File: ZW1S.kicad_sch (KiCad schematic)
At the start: 0 parts

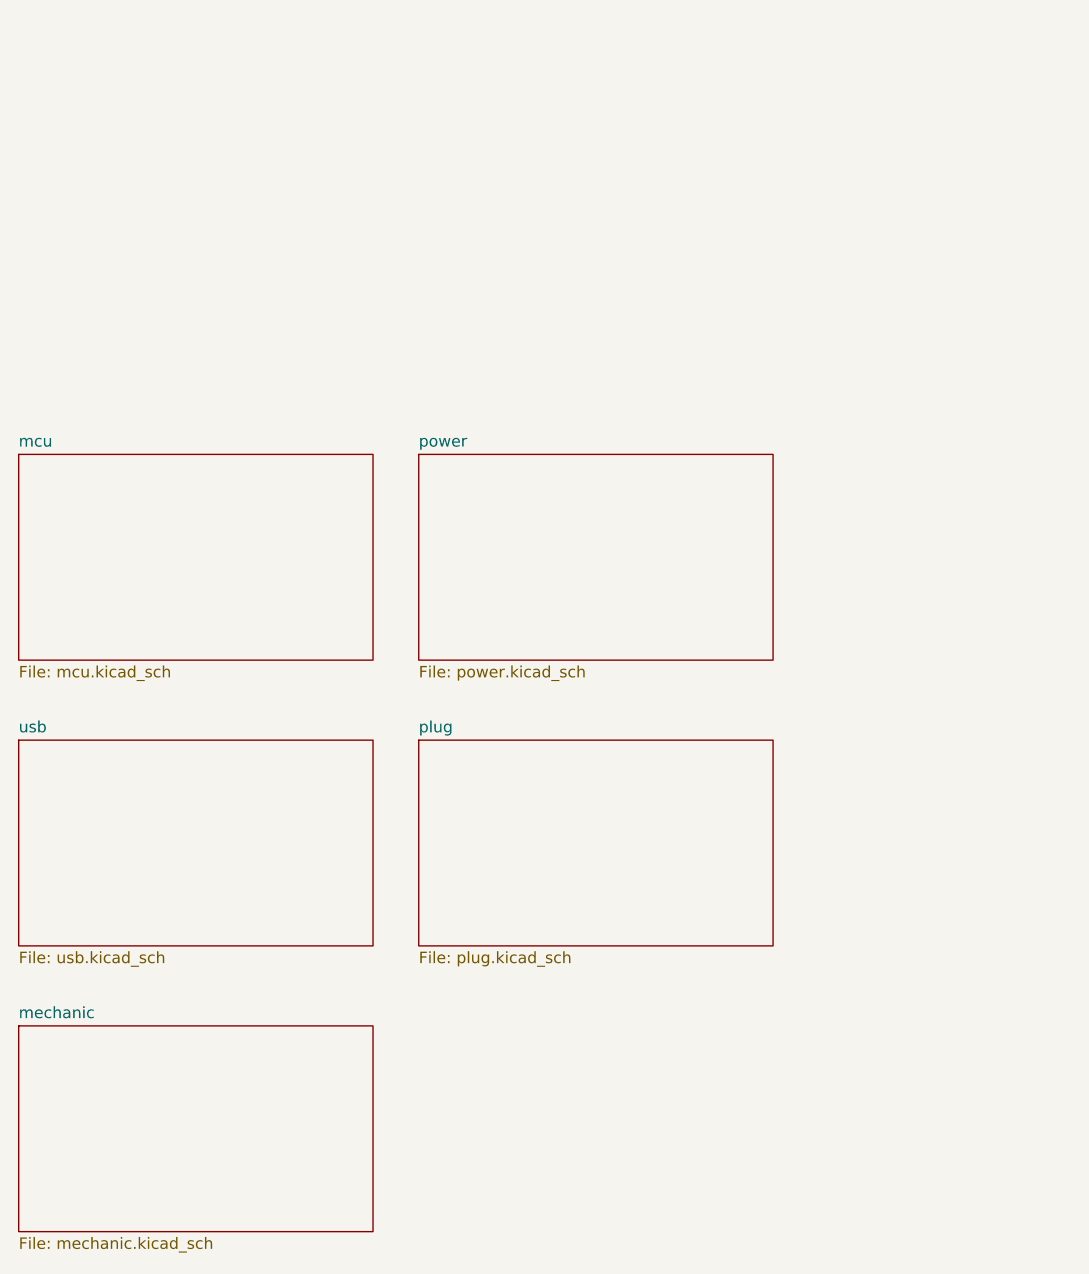
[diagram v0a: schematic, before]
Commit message: 暂存: 基本完成原理图(差雷达接口)
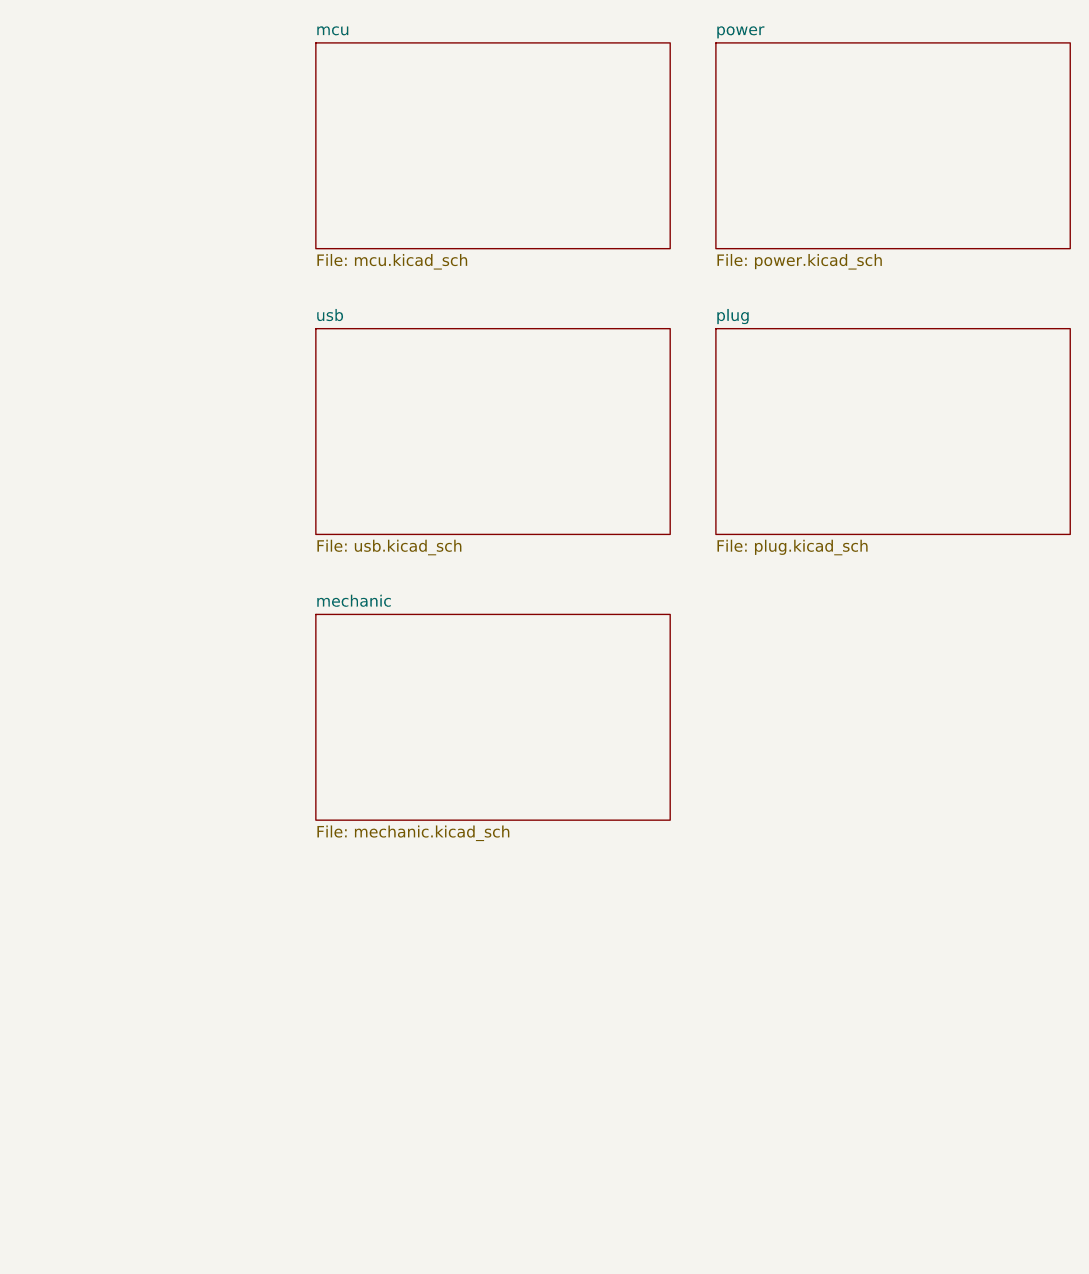
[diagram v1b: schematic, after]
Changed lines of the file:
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@@
 	(paper "A4")
 	(sheet
-		(at 30.48 156.21)
+		(at 63.5 110.49)
 		(size 39.37 22.86)
 		(fields_autoplaced yes)
@@
 		)
 		(property "Sheetname" "mechanic"
-			(at 30.48 155.4984 0)
+			(at 63.5 109.7784 0)
 			(effects
 				(font
@@
 		)
 		(property "Sheetfile" "mechanic.kicad_sch"
-			(at 30.48 179.6546 0)
+			(at 63.5 133.9346 0)
 			(effects
 				(font
@@
 	)
 	(sheet
-		(at 74.93 92.71)
+		(at 107.95 46.99)
 		(size 39.37 22.86)
 		(fields_autoplaced yes)
@@
 		)
 		(property "Sheetname" "power"
-			(at 74.93 91.9984 0)
+			(at 107.95 46.2784 0)
 			(effects
 				(font
@@
 		)
 		(property "Sheetfile" "power.kicad_sch"
-			(at 74.93 116.1546 0)
+			(at 107.95 70.4346 0)
 			(effects
 				(font
@@
 	)
 	(sheet
-		(at 30.48 92.71)
+		(at 63.5 46.99)
 		(size 39.37 22.86)
 		(fields_autoplaced yes)
@@
 		)
 		(property "Sheetname" "mcu"
-			(at 30.48 91.9984 0)
+			(at 63.5 46.2784 0)
 			(effects
 				(font
@@
 		)
 		(property "Sheetfile" "mcu.kicad_sch"
-			(at 30.48 116.1546 0)
+			(at 63.5 70.4346 0)
 			(effects
 				(font
@@
 	)
 	(sheet
-		(at 30.48 124.46)
+		(at 63.5 78.74)
 		(size 39.37 22.86)
 		(fields_autoplaced yes)
@@
 		)
 		(property "Sheetname" "usb"
-			(at 30.48 123.7484 0)
+			(at 63.5 78.0284 0)
 			(effects
 				(font
@@
 		)
 		(property "Sheetfile" "usb.kicad_sch"
-			(at 30.48 147.9046 0)
+			(at 63.5 102.1846 0)
 			(effects
 				(font
@@
 	)
 	(sheet
-		(at 74.93 124.46)
+		(at 107.95 78.74)
 		(size 39.37 22.86)
 		(fields_autoplaced yes)
@@
 		)
 		(property "Sheetname" "plug"
-			(at 74.93 123.7484 0)
+			(at 107.95 78.0284 0)
 			(effects
 				(font
@@
 		)
 		(property "Sheetfile" "plug.kicad_sch"
-			(at 74.93 147.9046 0)
+			(at 107.95 102.1846 0)
 			(effects
 				(font
